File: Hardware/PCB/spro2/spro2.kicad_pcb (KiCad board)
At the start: 2 copper layers, 100 x 60 mm, 46 parts, among them J2 MAX30102, J3 Humidity sensor, U1 LM35-LP, U2 OPA340P, U3 TL074

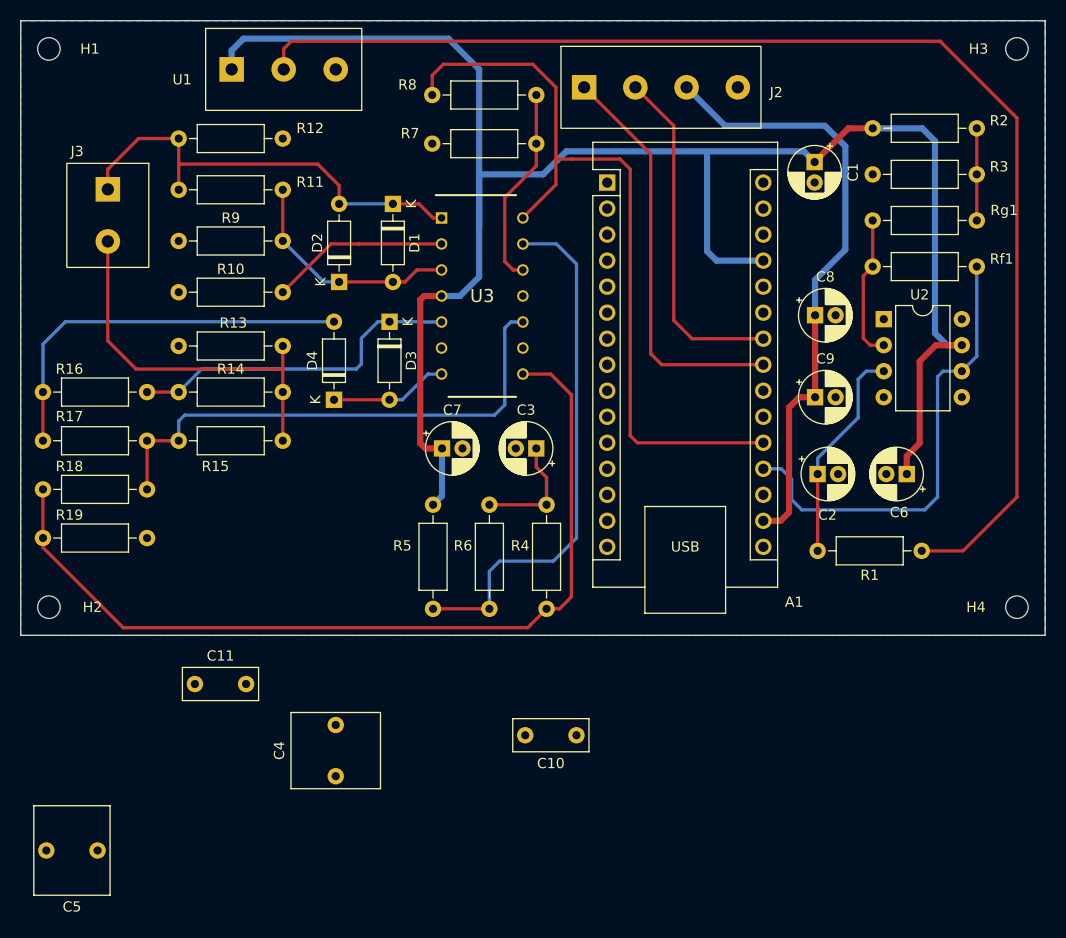
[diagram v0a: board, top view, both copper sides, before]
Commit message: Hopefully last version of PCB
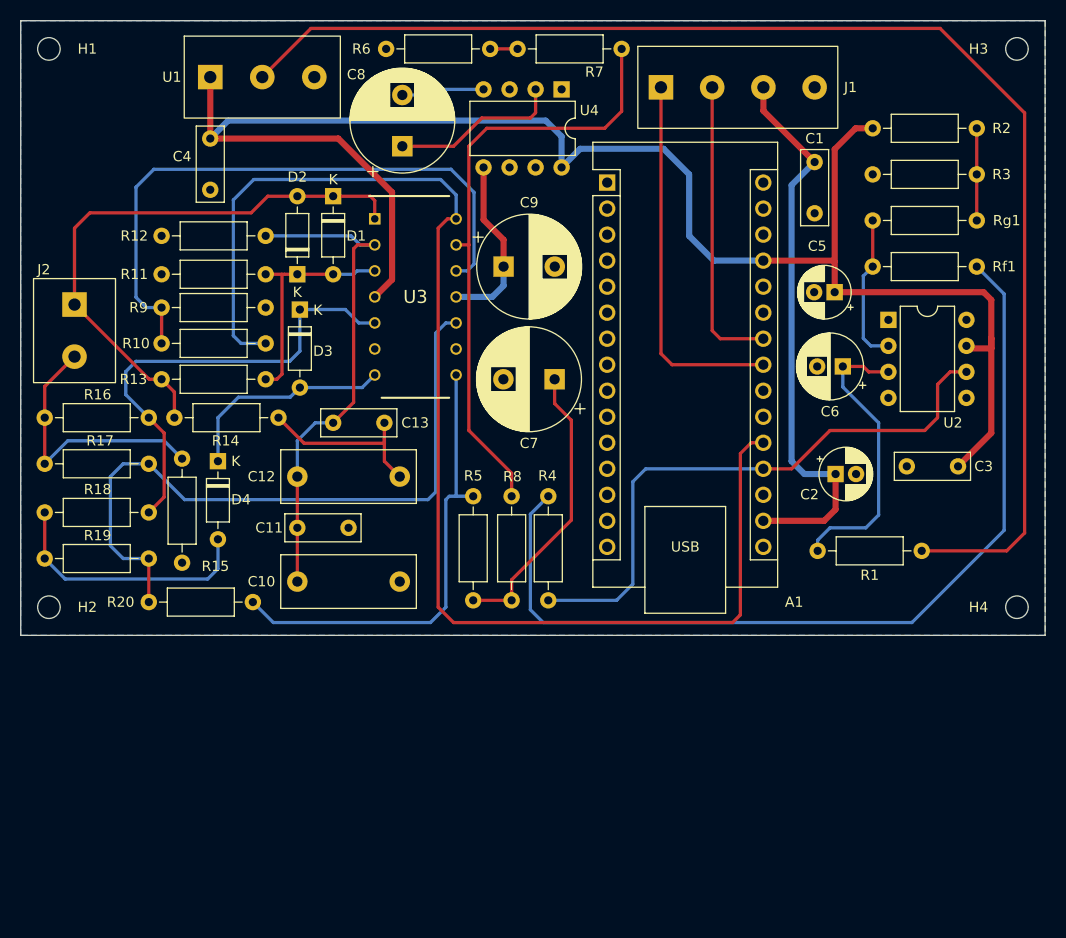
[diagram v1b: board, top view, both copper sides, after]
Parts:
- removed J3: Humidity sensor, Diplomna:connector_2p
- added C12: 1.5u, Capacitor_THT:C_Rect_L13.0mm_W5.0mm_P10.00mm_FKS3_FKP3_MKS4, F.Cu at (112.0, 123.8)
- added C13: 100n, Capacitor_THT:C_Rect_L7.2mm_W2.5mm_P5.00mm_FKS2_FKP2_MKS2_MKP2, F.Cu at (110.5, 118.5)
- added J1: MAX30102, Diplomna:connector_4p, F.Cu at (147.5, 85.8)
- added R20: 200k, Resistor_THT:R_Axial_DIN0207_L6.3mm_D2.5mm_P10.16mm_Horizontal, F.Cu at (87.5, 136.0)
- added U4: ~, Package_DIP:DIP-8_W7.62mm, F.Cu at (127.8, 86.0)
- C1: value 4.7µF -> 100n; footprint Capacitor_THT:CP_Radial_D5.0mm_P2.00mm -> Capacitor_THT:C_Rect_L7.2mm_W2.5mm_P5.00mm_FKS2_FKP2_MKS2_MKP2
- C10: value 100n -> 1.5u; footprint Capacitor_THT:C_Rect_L7.2mm_W3.0mm_P5.00mm_FKS2_FKP2_MKS2_MKP2 -> Capacitor_THT:C_Rect_L13.0mm_W5.0mm_P10.00mm_FKS3_FKP3_MKS4
- C11: footprint Capacitor_THT:C_Rect_L7.2mm_W3.0mm_P5.00mm_FKS2_FKP2_MKS2_MKP2 -> Capacitor_THT:C_Rect_L7.2mm_W2.5mm_P5.00mm_FKS2_FKP2_MKS2_MKP2
- C2: value 2.2u -> 4.7µF
- C3: value 4.7u -> 100n; footprint Capacitor_THT:CP_Radial_D5.0mm_P2.00mm -> Capacitor_THT:C_Rect_L7.2mm_W2.5mm_P5.00mm_FKS2_FKP2_MKS2_MKP2
- C4: value 1.5u -> 100n; footprint Capacitor_THT:C_Rect_L7.2mm_W8.5mm_P5.00mm_FKP2_FKP2_MKS2_MKP2 -> Capacitor_THT:C_Rect_L7.2mm_W2.5mm_P5.00mm_FKS2_FKP2_MKS2_MKP2
- C5: value 1.5u -> 4.7µF; footprint Capacitor_THT:C_Rect_L7.2mm_W8.5mm_P5.00mm_FKP2_FKP2_MKS2_MKP2 -> Capacitor_THT:CP_Radial_D5.0mm_P2.00mm
- C6: value 100n -> 2.2u; footprint Capacitor_THT:CP_Radial_D5.0mm_P2.00mm -> Capacitor_THT:CP_Radial_D6.3mm_P2.50mm
- C7, C9: value 100n -> 100u; footprint Capacitor_THT:CP_Radial_D5.0mm_P2.00mm -> Capacitor_THT:CP_Radial_D10.0mm_P5.00mm
- C8: value 4.7µF -> 100u; footprint Capacitor_THT:CP_Radial_D5.0mm_P2.00mm -> Capacitor_THT:CP_Radial_D10.0mm_P5.00mm
- J2: value MAX30102 -> Humidity sensor; footprint Diplomna:connector_4p -> Diplomna:connector_2p
- R10: value 100 -> 43k
- R11: value 240 -> 100
- R13: value 47k -> 240
- R14: value 1k -> 100
- R15: value 1k -> 47k
- R16, R18: value 1k -> 200k
- R17: value 500 -> 200k
- R19: value 10k -> 100k
- R3: value 270 -> 240
- R4: value 3.3 -> 10k
- R5: value 91k -> 200
- R6: value 1k -> 22k
- R7: value 10k -> 91k
- R8: value 33k -> 1k
- R9: value 100 -> 10k
- moved C5 90.3 mm to (154.5, 105.8)
- moved J2 64.3 mm to (80.2, 109.5), turned to -90 degrees
- moved C4 63.4 mm to (93.5, 90.8), turned to -90 degrees
- moved R8 49.4 mm to (122.9, 135.8), turned to 90 degrees
- moved R6 45.6 mm to (110.7, 82.0), turned to 0 degrees
- moved C8 43.5 mm to (112.2, 91.5), turned to 90 degrees
- moved C3 41.2 mm to (166.5, 122.8)
- moved C9 33.0 mm to (122.1, 103.2)
- moved C10 31.1 mm to (102.0, 134.0), turned to 0 degrees
- moved C11 18.2 mm to (102.0, 128.8)
- moved R12 15.2 mm to (88.8, 100.2), turned to 0 degrees
- moved R11 14.4 mm to (88.8, 104.0), turned to 0 degrees
- moved C7 12.9 mm to (127.1, 114.2), turned to 180 degrees
- moved D4 12.8 mm to (94.2, 122.2), turned to -90 degrees
- moved R7 12.4 mm to (123.5, 82.0)
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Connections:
- C1 pad 1: +5V -> +3.3V
- C11 pad 1: Net-(C11-Pad1) -> Net-(U3A--)
- C11 pad 2: Net-(U3A--) -> GND
- C2 pad 1: Net-(U2-+) -> +3.3V
- C3 pad 1: Net-(C3-Pad1) -> +5V
- C4 pad 1: Net-(U3A--) -> +5V
- C5 pad 1: Net-(C11-Pad1) -> +5V
- C5 pad 2: Net-(U3A--) -> GND
- C6 pad 1: +5V -> Net-(U2-+)
- C7 pad 1: +5V -> Net-(C7-Pad1)
- C8 pad 1: +3.3V -> Net-(U4-CAP+)
- C8 pad 2: GND -> Net-(U4-CAP-)
- C9 pad 1: +3.3V -> -5V
- J2 pad 1: Net-(A1-A4) -> Net-(D1-K)
- J2 pad 2: Net-(A1-A5) -> Net-(J2-Pin_2)
- R10 pad 1: GND -> Net-(U3D-+)
- R10 pad 2: Net-(U3A--) -> /Humidity
- R11 pad 1: Net-(D1-A) -> GND
- R11 pad 2: Net-(D1-K) -> Net-(D1-A)
- R12 pad 1: Net-(C11-Pad1) -> GND
- R12 pad 2: Net-(D1-K) -> Net-(U3A--)
- R13 pad 1: Net-(J3-Pin_2) -> Net-(D1-A)
- R13 pad 2: GND -> Net-(D1-K)
- R14 pad 1: Net-(J3-Pin_2) -> Net-(C12-Pad1)
- R14 pad 2: Net-(D3-K) -> Net-(D1-K)
- R15 pad 1: Net-(J3-Pin_2) -> Net-(J2-Pin_2)
- R15 pad 2: Net-(U3C-+) -> GND
- R16 pad 1: Net-(D3-K) -> Net-(J2-Pin_2)
- R16 pad 2: Net-(D4-A) -> Net-(D3-K)
- R17 pad 1: Net-(D4-A) -> Net-(J2-Pin_2)
- R18 pad 1: Net-(U3C-+) -> Net-(D3-K)
- R18 pad 2: /Humidity Amplifier/Humidity_In -> Net-(D4-A)
- R19 pad 1: /Humidity Amplifier/Humidity_In -> Net-(D4-A)
- R19 pad 2: GND -> Net-(U3C-+)
- R4 pad 1: /Humidity Amplifier/Humidity_In -> /Temp
- R4 pad 2: Net-(C3-Pad1) -> Net-(R4-Pad2)
- R5 pad 1: +5V -> /Humidity Amplifier/Humidity_In
- R5 pad 2: Net-(U3D--) -> Net-(C7-Pad1)
- R6 pad 1: Net-(C3-Pad1) -> GND
- R6 pad 2: Net-(U3D--) -> Net-(R6-Pad2)
- R7 pad 1: GND -> Net-(R6-Pad2)
- R7 pad 2: Net-(U3D-+) -> Net-(U3D--)
- R8 pad 1: Net-(U3D-+) -> Net-(C7-Pad1)
- R8 pad 2: /Humidity -> Net-(U3D--)
- R9 pad 2: Net-(D1-A) -> Net-(U3D-+)
- Rf1 pad 2: /Temp -> Net-(R4-Pad2)
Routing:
- net Net-(R4-Pad2): track 0.00 -> 89.2 mm
- net /Humidity: track 76.4 -> 130.2 mm
- net /Humidity Amplifier/Humidity_In: track 87.1 -> 45.4 mm
- net Net-(U3D-+): track 19.6 -> 60.8 mm
- net Net-(J3-Pin_2): track 37.2 -> 0.00 mm
- net Net-(U3A--): track 17.5 -> 49.0 mm
- net Net-(C7-Pad1): track 0.00 -> 28.4 mm
- net Net-(J2-Pin_2): track 0.00 -> 26.7 mm
- net Net-(C12-Pad1): track 0.00 -> 18.2 mm
- net -5V: track 0.00 -> 17.4 mm
- net +5V: track 183.4 -> 166.1 mm
- net Net-(U4-CAP+): track 0.00 -> 16.7 mm
- net Net-(U3C-+): track 51.8 -> 67.2 mm
- net Net-(D4-A): track 38.7 -> 25.5 mm
- net Net-(D3-K): track 33.1 -> 45.7 mm
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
